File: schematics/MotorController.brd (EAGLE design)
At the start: 121.9 x 93.7 mm, 40 parts, among them IC1 7805, Q1 BC307

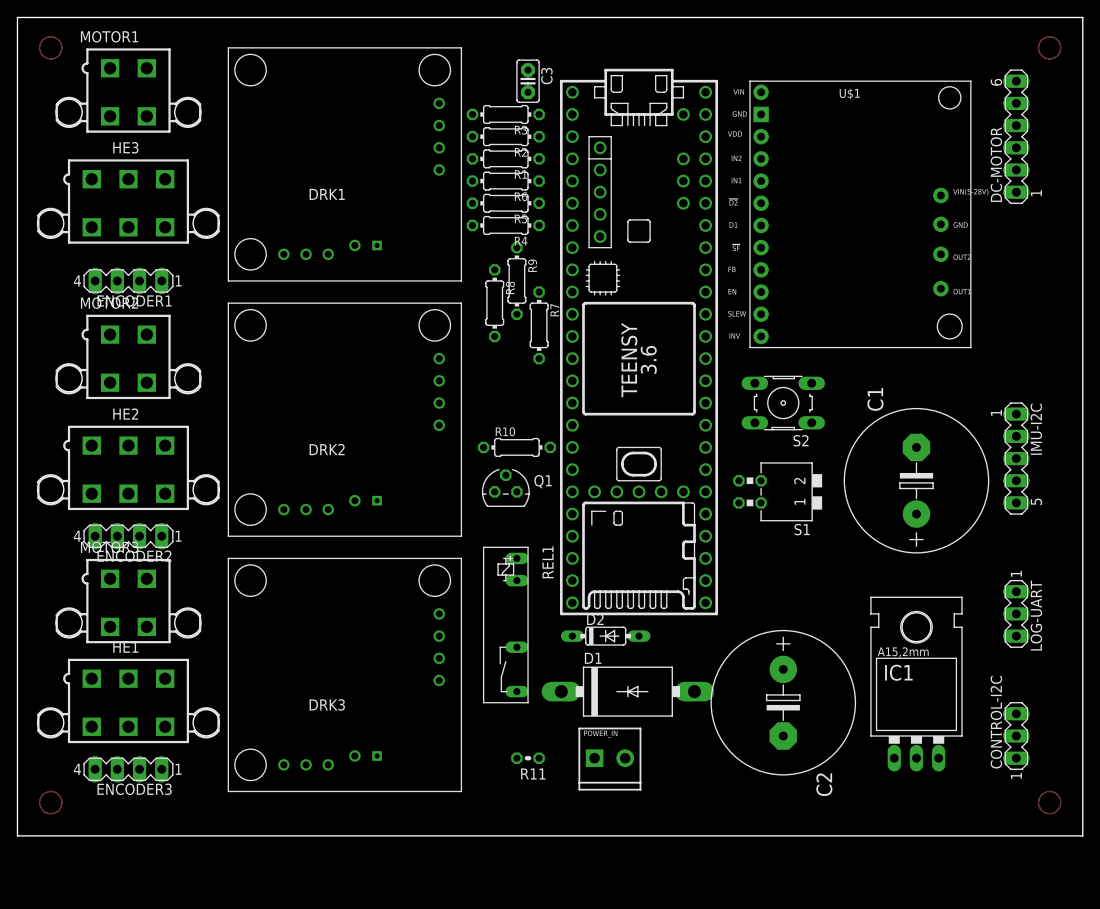
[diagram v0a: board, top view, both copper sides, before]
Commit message: no message
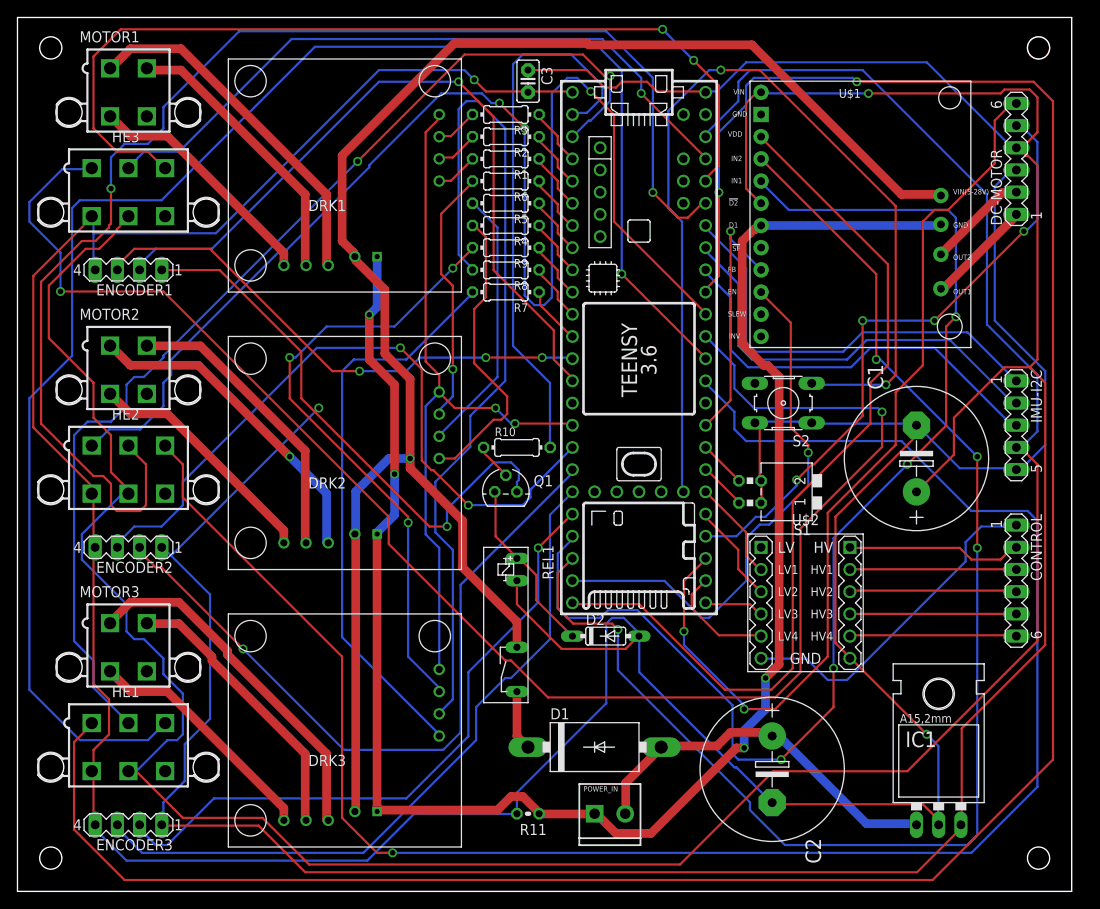
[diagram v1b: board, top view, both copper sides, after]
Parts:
- removed CONTROL-I2C, LOG-UART: 1, con-lstb:MA03-1
- added CONTROL: (no value), con-lstb:MA06-1
- added U$2: LEVEL-SHIFTER-4CHLEVEL-SHIFTER-4CH-ADAFRUIT, diy-modules:LEVEL-SHIFTER-4CH-ADAFRUIT
- moved IC1 8.03 mm to (30.5, -2.54)
- moved C2 7.73 mm to (11.4, 0.00)
- moved D1 7.41 mm to (-8.89, 2.54)
- moved DRK3 6.35 mm to (-38.1, 5.08)
- moved ENCODER3 6.35 mm to (-62.2, -6.35)
- moved POWER_IN 6.35 mm to (-8.89, -5.08)
- moved R11 6.35 mm to (-16.5, -5.08)
- moved R7 5.39 mm to (-19.1, 54.6), turned to 180 degrees
- moved HE1 5.08 mm to (-62.2, 2.54)
- moved MOTOR3 5.08 mm to (-62.2, 14.0)
- moved R8 4.02 mm to (-19.1, 57.1), turned to 180 degrees
- moved R9 4.02 mm to (-19.1, 59.7), turned to 180 degrees
- moved DRK2 3.81 mm to (-38.1, 36.8)
- moved IMU-I2C 3.81 mm to (39.4, 39.4)
- moved DC-MOTOR 2.54 mm to (39.4, 69.8)
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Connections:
- removed net CTRL-SDA: CONTROL-I2C.1, PRJ1.37/A18
- removed net N$43: CONTROL-I2C.2, PRJ1.38/A19
- removed net N$53: HE1.5, HE2.5, HE3.5
- new net LCTR-VDD: CONTROL.6, U$2.HV4
- new net LCTRL-GND: CONTROL.1, U$2.GNDL
- new net LCTRL-RX: CONTROL.5, U$2.HV3
- new net LCTRL-SCL: CONTROL.4, U$2.HV2
- new net LCTRL-SDA: CONTROL.3, U$2.HV1
- new net LCTRL-VDD: CONTROL.2, U$2.HV
- new net LV: U$2.LV
- new net N$60: PRJ1.A22/DAC1, U$1.FB
- new net SCL1: PRJ1.38/A19, U$2.LV1
- new net SDA1: PRJ1.37/A18, U$2.LV2
- net GND: now also PRJ1.AGND, PRJ1.GND2, U$2.GNDH; no longer CONTROL-I2C.3, LOG-UART.3
- net LIPO-GND: now also U$1.D1
- net N$46: now also HE1.5, HE2.5, HE3.5
- net RX5: now also U$2.LV4; no longer LOG-UART.1
- net TX5: now also U$2.LV3; no longer LOG-UART.2
- net VCC: now also U$1.!D2
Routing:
- net VCC: track 0.00 -> 442.4 mm, vias 0 -> 3
- net GND: track 0.00 -> 432.3 mm, vias 0 -> 2
- net N$46: track 0.00 -> 301.9 mm
- net N$54: track 0.00 -> 270.7 mm, vias 0 -> 2
- net N$59: track 0.00 -> 211.8 mm, vias 0 -> 1
- net LIPO-GND: track 0.00 -> 199.6 mm, vias 0 -> 4
- net LIPO-VDD: track 0.00 -> 190.2 mm, vias 0 -> 1
- net N$56: track 0.00 -> 186.4 mm, vias 0 -> 2
- net N$58: track 0.00 -> 184.5 mm, vias 0 -> 1
- net N$47: track 0.00 -> 157.2 mm, vias 0 -> 4
- net N$55: track 0.00 -> 153.8 mm, vias 0 -> 3
- net N$51: track 0.00 -> 152.9 mm, vias 0 -> 2
- net N$44: track 0.00 -> 140.1 mm, vias 0 -> 4
- net N$57: track 0.00 -> 126.4 mm, vias 0 -> 2
- net N$52: track 0.00 -> 108.3 mm, vias 0 -> 2
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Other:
- board size 121.9 x 93.7 mm -> 120.6 x 100 mm

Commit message: ordered PCB
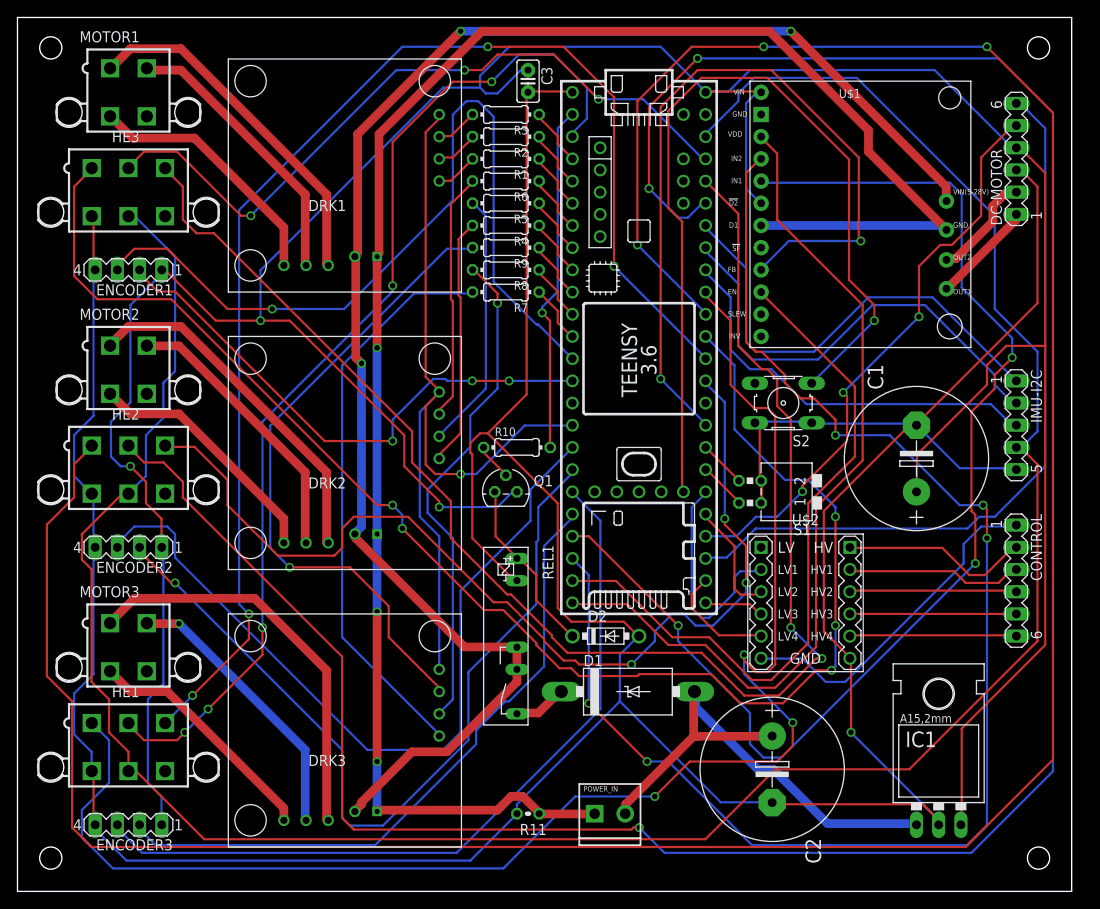
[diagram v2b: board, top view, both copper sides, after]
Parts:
- D1: value 1N5400 -> 1N5908; device diode:DO201-15 -> diode:C4111-15
- D2: value 1N4148DO35-7 -> 1N5818-B; device diode:DO35-7 -> diode:DO41-7.6
- moved D1 7.41 mm to (-5.08, 8.89)
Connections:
- net GND: no longer PRJ1.AGND, PRJ1.GND2
- net LIPO-VDD: now also REL1.5
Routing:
- net N$55: track 153.8 -> 319.2 mm
- net N$51: track 152.9 -> 285.4 mm, vias 2 -> 3
- net N$54: track 270.7 -> 168.5 mm, vias 2 -> 3
- net N$59: track 211.8 -> 115.1 mm, vias 1 -> 3
- net VCC: track 442.4 -> 372.5 mm
- net N$50: track 105.5 -> 169.4 mm
- net N$60: track 29.2 -> 89.6 mm, vias 1 -> 2
- net N$24: track 97.8 -> 57.2 mm, vias 0 -> 1
- net N$33: track 59.8 -> 95.0 mm, vias 3 -> 1
- net N$58: track 184.5 -> 150.4 mm, vias 1 -> 4
- net N$42: track 63.4 -> 40.0 mm, vias 0 -> 1
- net N$34: track 85.4 -> 62.4 mm, vias 1 -> 3
- net WH_ENC_B: track 106.7 -> 86.4 mm, vias 2 -> 0
- net N$45: track 62.2 -> 80.2 mm, vias 1 -> 0
- net N$56: track 186.4 -> 169.0 mm, vias 2 -> 5
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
